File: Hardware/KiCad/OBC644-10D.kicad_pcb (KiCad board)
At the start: 2 copper layers, 45 x 45 mm, 62 parts, among them J1 CONN_11, J2 CONN_11, J3 CONN_4, J4 CONN_6, J5 CONN_2, U1 LT1761ES5-3.3, U10 LT1761ES5-xx, U11 LT1761ES5-xx, U12 M25P80, U2 ATMEGA644PA-A, U3 REF3320, U4 RX8900CE, U5 MS5611, U6 MPU-9250, U7 microSD_hinge, U8 M25P80, U9 INA226, X1 CRYSTAL

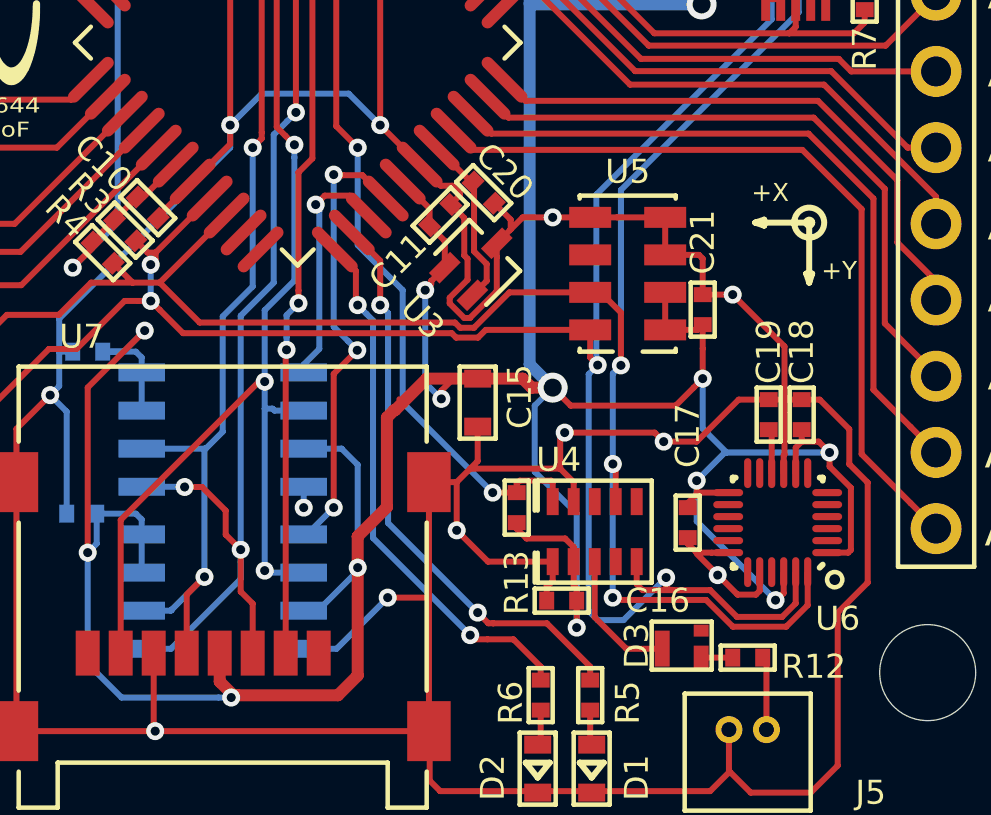
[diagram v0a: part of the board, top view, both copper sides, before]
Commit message: fix spacing
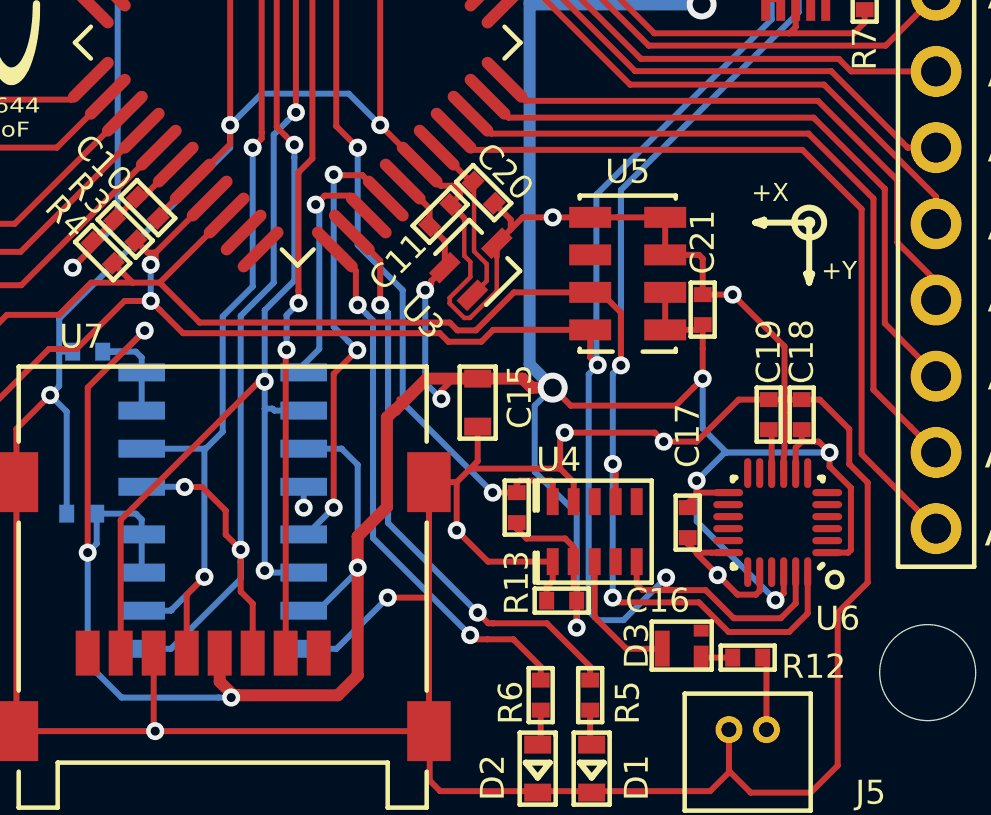
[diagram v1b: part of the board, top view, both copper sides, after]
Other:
- rule trace_min: 0.127 -> 0.15
